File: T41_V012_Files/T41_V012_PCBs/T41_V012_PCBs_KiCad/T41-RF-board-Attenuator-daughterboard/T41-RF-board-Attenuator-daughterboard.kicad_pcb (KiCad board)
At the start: 2 copper layers, 13.7 x 16.3 mm, 6 parts, among them J1 Conn 1, J2 Conn 2, U1 PE4312

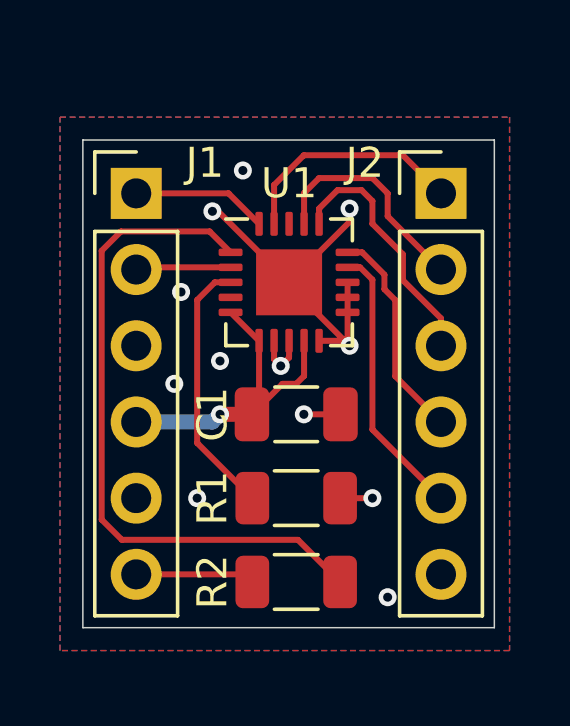
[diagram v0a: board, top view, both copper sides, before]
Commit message: H1 removed and some via transitions removed for reduced EMI
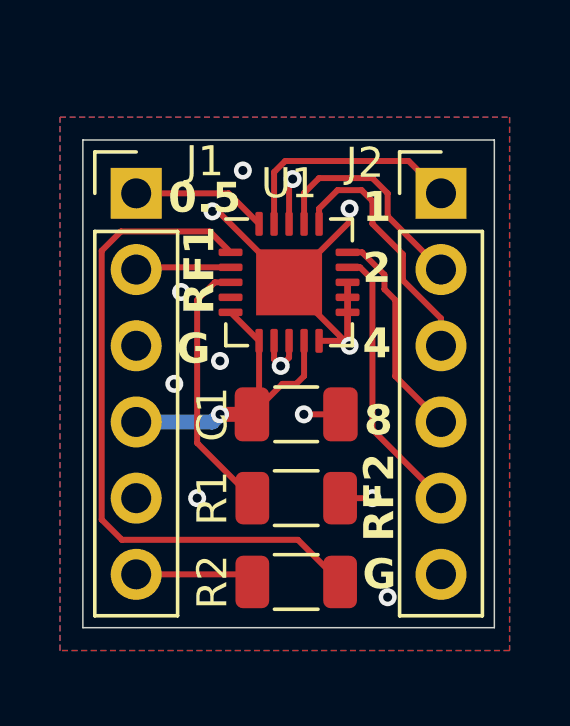
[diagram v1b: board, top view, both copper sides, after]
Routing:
- net GND: track 17.2 -> 20.8 mm, vias 12 -> 13
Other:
- board text added: "G"
- board text added: "RF1"
- board text added: "RF2"
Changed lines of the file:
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@@
 		(tags "Through hole pin header THT 1x06 2.54mm single row")
 		(property "Reference" "J1"
-			(at 2.286 -1.016 0)
+			(at 2.286 -1.0668 0)
 			(layer "F.SilkS")
 			(effects
@@
 		(layer "Edge.Cuts")
 	)
+	(gr_text "4"
+		(at 91.3638 69.088 0)
+		(layer "F.SilkS")
+		(effects
+			(font
+				(size 1 1)
+				(thickness 0.2)
+				(bold yes)
+			)
+			(justify left bottom)
+		)
+	)
+	(gr_text "RF2"
+		(at 92.5068 75.1078 90)
+		(layer "F.SilkS")
+		(effects
+			(font
+				(size 1 1)
+				(thickness 0.2)
+				(bold yes)
+			)
+			(justify left bottom)
+		)
+	)
+	(gr_text "0.5"
+		(at 84.8868 64.2366 0)
+		(layer "F.SilkS")
+		(effects
+			(font
+				(size 1 1)
+				(thickness 0.2)
+				(bold yes)
+			)
+			(justify left bottom)
+		)
+	)
+	(gr_text "G"
+		(at 91.3638 76.7842 0)
+		(layer "F.SilkS")
+		(effects
+			(font
+				(size 1 1)
+				(thickness 0.2)
+				(bold yes)
+			)
+			(justify left bottom)
+		)
+	)
+	(gr_text "2"
+		(at 91.3638 66.5734 0)
+		(layer "F.SilkS")
+		(effects
+			(font
+				(size 1 1)
+				(thickness 0.2)
+				(bold yes)
+			)
+			(justify left bottom)
+		)
+	)
+	(gr_text "8"
+		(at 91.4146 71.6534 0)
+		(layer "F.SilkS")
+		(effects
+			(font
+				(size 1 1)
+				(thickness 0.2)
+				(bold yes)
+			)
+			(justify left bottom)
+		)
+	)
+	(gr_text "1"
+		(at 91.3638 64.5414 0)
+		(layer "F.SilkS")
+		(effects
+			(font
+				(size 1 1)
+				(thickness 0.2)
+				(bold yes)
+			)
+			(justify left bottom)
+		)
+	)
+	(gr_text "G"
+		(at 85.1662 69.2658 0)
+		(layer "F.SilkS")
+		(effects
+			(font
+				(size 1 1)
+				(thickness 0.2)
+				(bold yes)
+			)
+			(justify left bottom)
+		)
+	)
+	(gr_text "RF1"
+		(at 86.5124 67.5386 90)
+		(layer "F.SilkS")
+		(effects
+			(font
+				(size 1 1)
+				(thickness 0.2)
+				(bold yes)
+			)
+			(justify left bottom)
+		)
+	)
 	(gr_text "T41 Att. Brd\nV1 27DEC25"
 		(at 91.186 61.976 90)
@@
 	)
 	(segment
+		(start 88.916 66.466)
+		(end 90.932 64.45)
+		(width 0.2)
+		(layer "F.Cu")
+		(net 2)
+	)
+	(segment
+		(start 86.55 64.1)
+		(end 86.36 64.1)
+		(width 0.2)
+		(layer "F.Cu")
+		(net 2)
+	)
+	(segment
+		(start 88.916 64.516)
+		(end 88.916 63.143471)
+		(width 0.2)
+		(layer "F.Cu")
+		(net 2)
+	)
+	(segment
+		(start 90.866 66.466)
+		(end 90.866 67.466)
+		(width 0.2)
+		(layer "F.Cu")
+		(net 2)
+	)
+	(segment
+		(start 88.916 63.143471)
+		(end 89.036171 63.0233)
+		(width 0.2)
+		(layer "F.Cu")
+		(net 2)
+	)
+	(segment
+		(start 88.416 69.031378)
+		(end 88.637393 69.252771)
+		(width 0.2)
+		(layer "F.Cu")
+		(net 2)
+	)
+	(segment
+		(start 90.768 68.416)
+		(end 90.932 68.58)
+		(width 0.2)
+		(layer "F.Cu")
+		(net 2)
+	)
+	(segment
 		(start 90.866 68.514)
 		(end 90.932 68.58)
@@
 	)
 	(segment
-		(start 88.916 66.466)
-		(end 90.932 64.45)
-		(width 0.2)
-		(layer "F.Cu")
-		(net 2)
-	)
-	(segment
-		(start 86.55 64.1)
-		(end 86.36 64.1)
-		(width 0.2)
-		(layer "F.Cu")
-		(net 2)
-	)
-	(segment
-		(start 90.866 66.466)
-		(end 90.866 67.466)
-		(width 0.2)
-		(layer "F.Cu")
-		(net 2)
-	)
-	(segment
-		(start 88.416 69.031378)
-		(end 88.637393 69.252771)
-		(width 0.2)
-		(layer "F.Cu")
-		(net 2)
-	)
-	(segment
-		(start 90.768 68.416)
-		(end 90.932 68.58)
-		(width 0.2)
-		(layer "F.Cu")
-		(net 2)
-	)
-	(segment
 		(start 88.416 68.416)
 		(end 88.416 69.031378)
@@
 		(start 88.916 66.564)
 		(end 90.932 68.58)
+		(width 0.2)
+		(layer "F.Cu")
+		(net 2)
+	)
+	(segment
+		(start 90.866 66.466)
+		(end 90.866 68.514)
 		(width 0.2)
 		(layer "F.Cu")
@@
 	)
 	(via
+		(at 89.036171 63.0233)
+		(size 0.6)
+		(drill 0.3)
+		(layers "F.Cu" "B.Cu")
+		(net 2)
+	)
+	(via
 		(at 92.202 76.962)
 		(size 0.6)
@@
 	)
 	(segment
-		(start 92.71 62.23)
+		(start 88.416 64.516)
+		(end 88.416 62.793528)
+		(width 0.2)
+		(layer "F.Cu")
+		(net 6)
+	)
+	(segment
+		(start 92.9023 62.4223)
 		(end 93.98 63.5)
 		(width 0.2)
@@
 	)
 	(segment
-		(start 88.416 64.516)
-		(end 88.416 63.222)
+		(start 88.416 62.793528)
+		(end 88.787228 62.4223)
 		(width 0.2)
 		(layer "F.Cu")
@@
 	)
 	(segment
-		(start 88.416 63.222)
-		(end 89.408 62.23)
-		(width 0.2)
-		(layer "F.Cu")
-		(net 6)
-	)
-	(segment
-		(start 89.408 62.23)
-		(end 92.71 62.23)
+		(start 88.787228 62.4223)
+		(end 92.9023 62.4223)
 		(width 0.2)
 		(layer "F.Cu")
@@
 	)
 	(zone
+		(net 0)
+		(net_name "")
+		(layer "F.Cu")
+		(hatch edge 0.5)
+		(connect_pads
+			(clearance 0)
+		)
+		(min_thickness 0.25)
+		(filled_areas_thickness no)
+		(keepout
+			(tracks allowed)
+			(vias allowed)
+			(pads allowed)
+			(copperpour not_allowed)
+			(footprints allowed)
+		)
+		(placement
+			(enabled no)
+			(sheetname "/")
+		)
+		(fill
+			(thermal_gap 0.5)
+			(thermal_bridge_width 0.5)
+		)
+		(polygon
+			(pts
+				(xy 87.376 64.9224) (xy 91.2622 64.9224) (xy 91.2876 68.0212) (xy 87.3506 68.0212)
+			)
+		)
+	)
+	(zone

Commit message: New layouts for RF board, clock board, and attenuator board are done
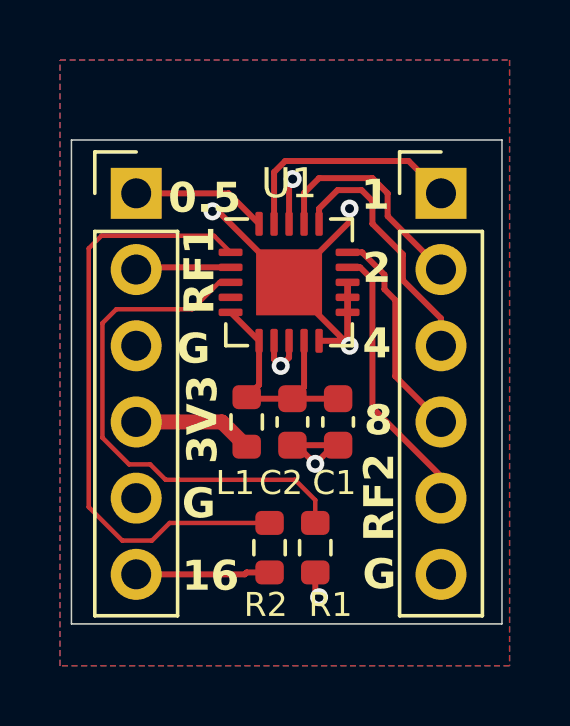
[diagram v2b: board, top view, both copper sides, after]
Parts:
- added C2: 10uF 50V, Capacitor_SMD:C_0603_1608Metric, F.Cu at (89.0, 71.1)
- added L1: FB, Resistor_SMD:R_0603_1608Metric, F.Cu at (87.5, 71.1)
- C1: footprint Capacitor_SMD:C_1206_3216Metric -> Capacitor_SMD:C_0603_1608Metric
- R1, R2: footprint Resistor_SMD:R_1206_3216Metric -> Resistor_SMD:R_0603_1608Metric
- moved R1 1.77 mm to (89.8, 75.3), turned to 90 degrees
- moved R2 1.45 mm to (88.3, 75.3), turned to -90 degrees
- moved C1 1.42 mm to (90.6, 71.1), turned to 90 degrees
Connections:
- C1 pad 2: +3V3 -> Net-(U1-LE)
- U1 pad 5: +3V3 -> Net-(U1-LE)
- U1 pad 6: +3V3 -> Net-(U1-LE)
- U1 pad 9: +3V3 -> Net-(U1-LE)
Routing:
- net Net-(U1-Data): track 8.72 -> 17.4 mm
- net Net-(U1-LE): track 0.00 -> 8.55 mm
- net +3V3: track 11.3 -> 4.02 mm, vias 1 -> 0
- net GND: track 20.8 -> 22.9 mm, vias 13 -> 7
- net Net-(U1-C16): track 22.6 -> 20.5 mm
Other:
- board size 13.7 x 16.3 mm -> 14.4 x 16.1 mm
